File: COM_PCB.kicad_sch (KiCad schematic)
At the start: 0 parts

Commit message: KiCad 0.3v
Improved aesthetics.
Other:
- sheet SI4463: file file5FC06DBC.kicad_sch -> UHF.kicad_sch

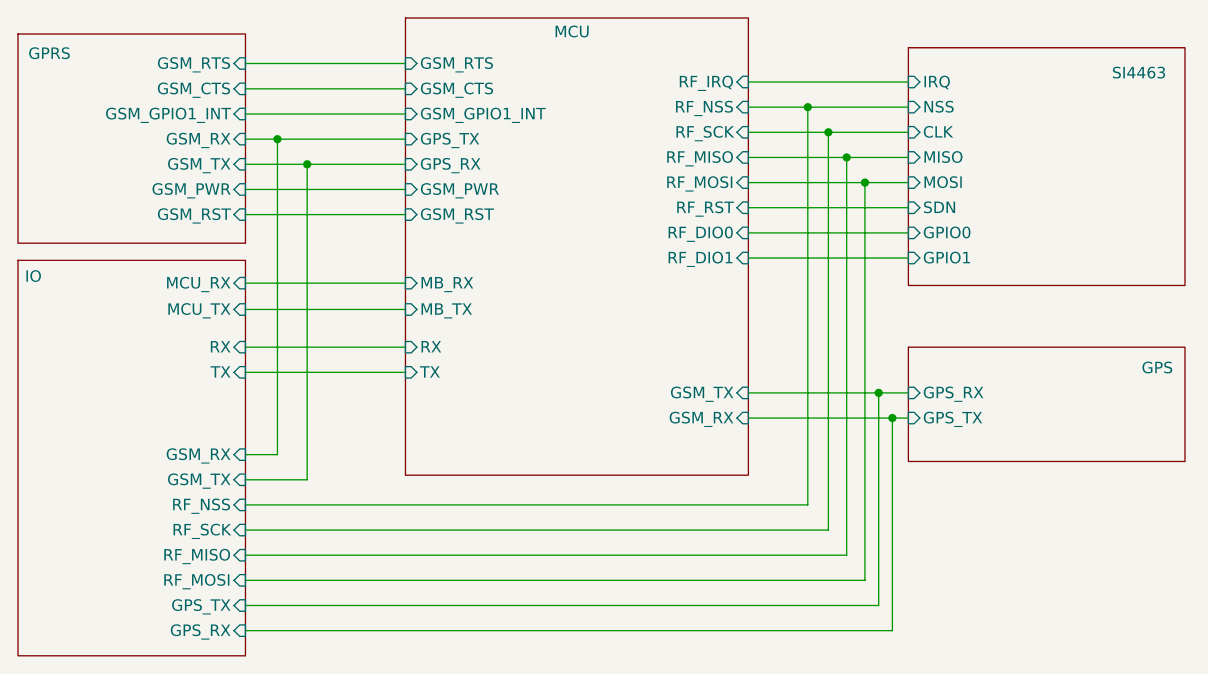
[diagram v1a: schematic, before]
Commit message: 0.1v COM_PCB KiCad
First iteration of COM PCB.
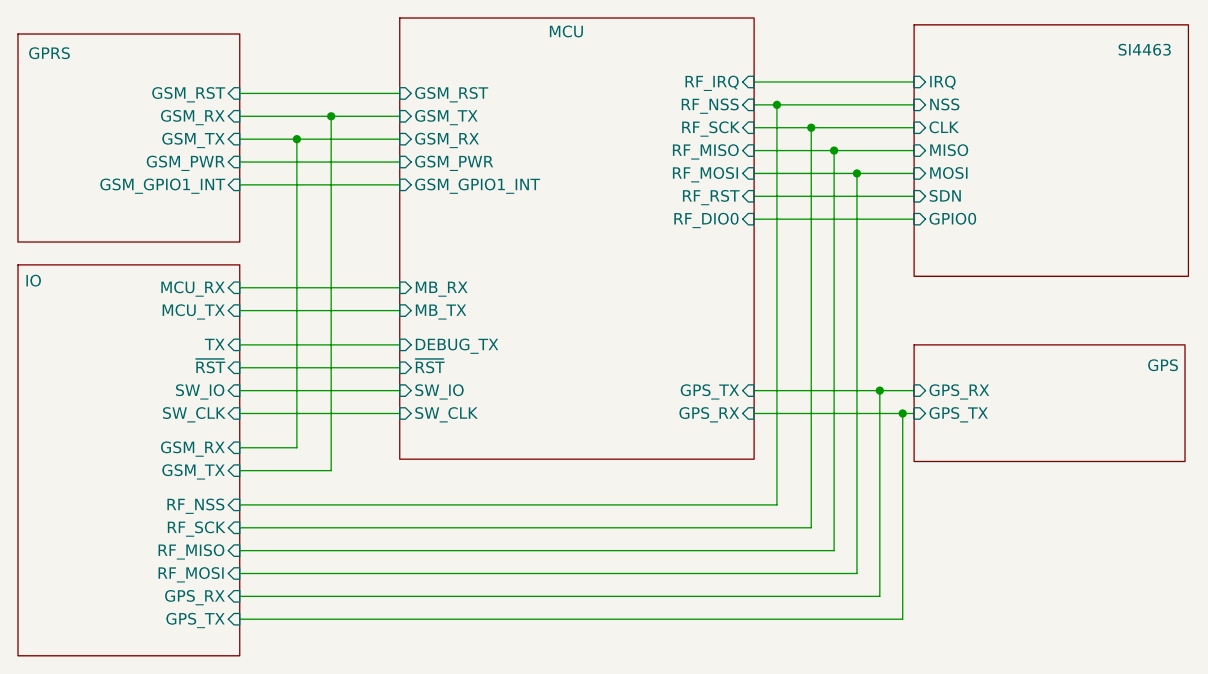
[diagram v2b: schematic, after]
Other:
- sheet GPRS ports: added none; removed GSM_CTS, GSM_RTS
- sheet IO ports: added SW_CLK, SW_IO, ~{RST}; removed RX
- sheet MCU ports: added DEBUG_TX, SW_CLK, SW_IO, ~{RST}; removed GSM_CTS, GSM_RTS, RF_DIO1, RX, TX
- sheet SI4463 ports: added none; removed GPIO1
